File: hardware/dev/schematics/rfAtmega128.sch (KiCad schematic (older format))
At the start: 6 parts

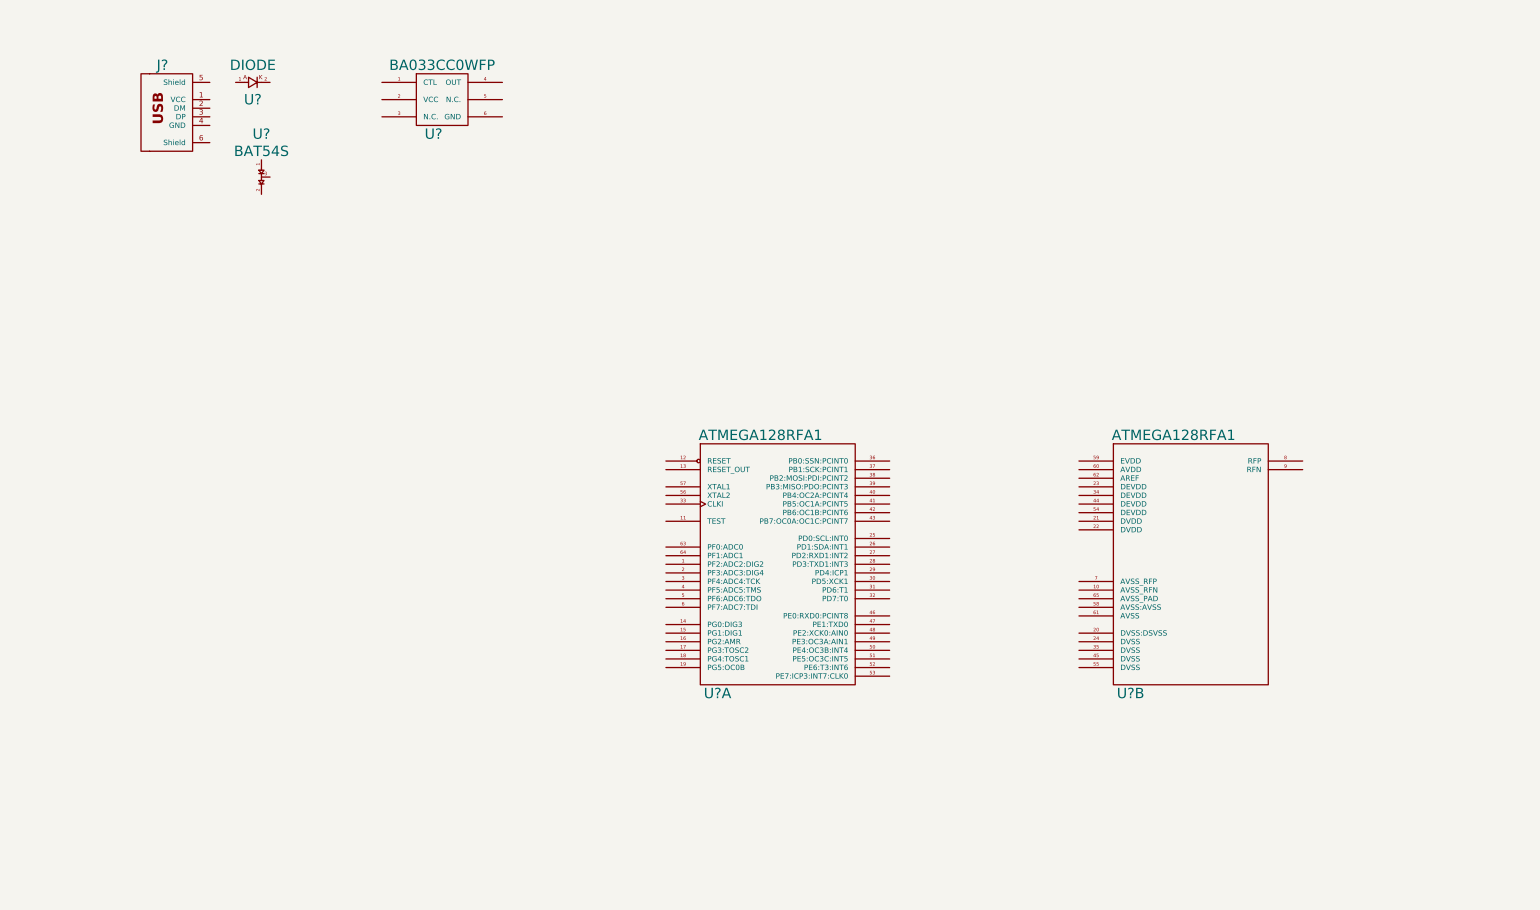
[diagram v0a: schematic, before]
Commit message: New schematic to finish at home.
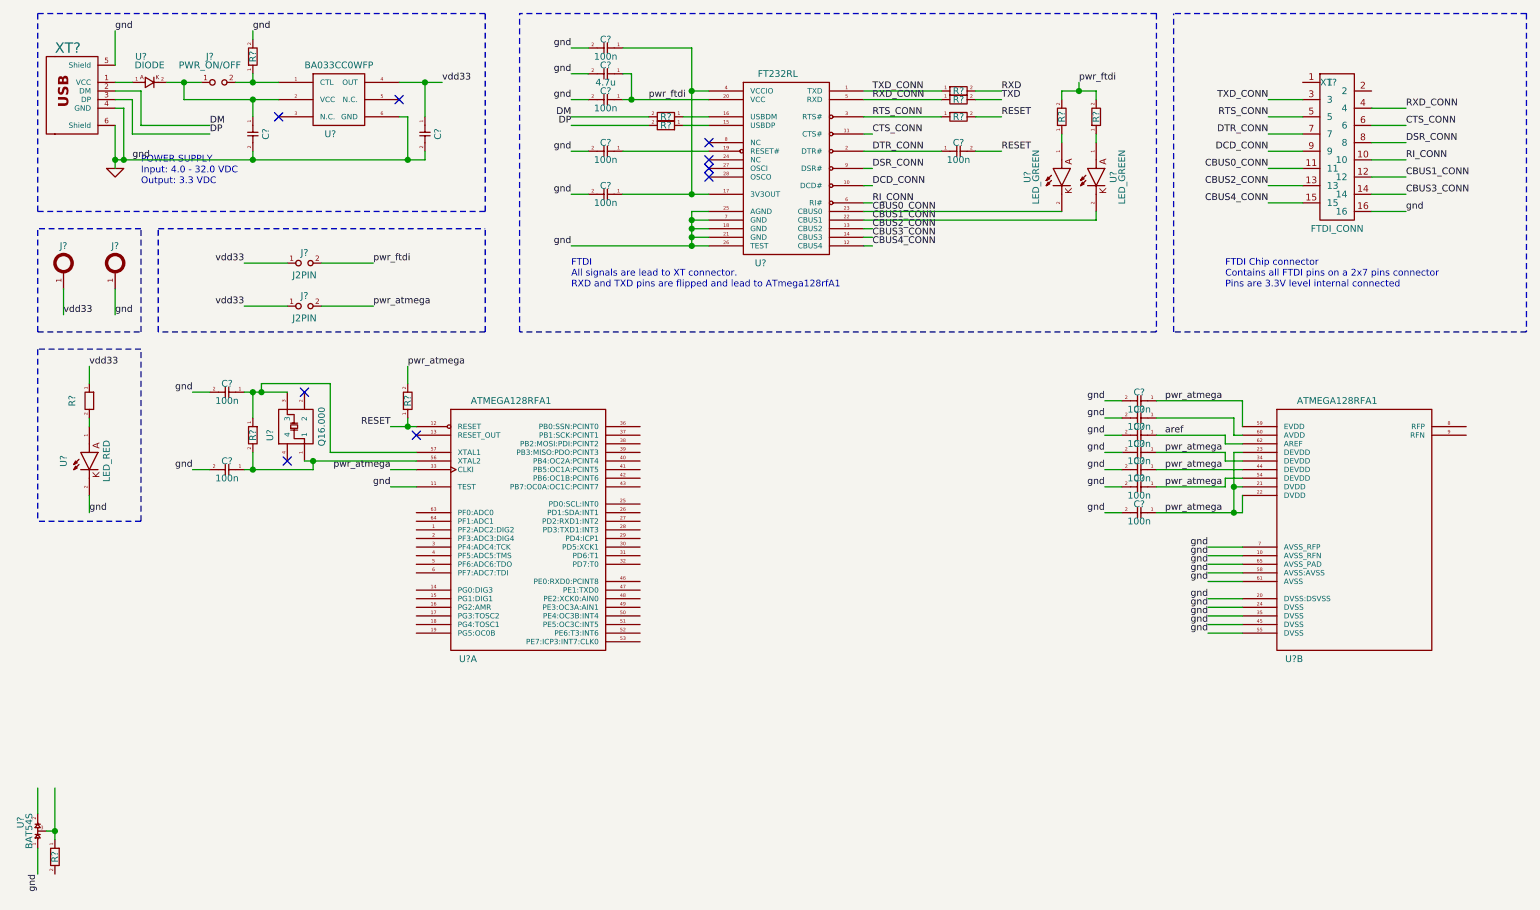
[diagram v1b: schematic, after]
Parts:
- added C?: 330n, symbol CAP_0603
- added C?: 22u, symbol CAP_0603
- added C? (x14): 100n, symbol CAP_0603
- added C?: 4.7u, symbol CAP_0603
- added J?: TEST_VDD33, symbol TEST_PAD
- added J?: TEST_GND, symbol TEST_PAD
- added J? (x2): J2PIN, symbol J2PIN
- added J?: PWR_ON/OFF, symbol J2PIN
- added R? (x12): RES_0603, symbol RES_0603
- added U?: FT232RL, symbol FT232RL
- added U?: LED_RED, symbol LED_RED
- added U? (x2): LED_GREEN, symbol LED_GREEN
- added U?: Q16.000, symbol Q16.000
- added XT?: FTDI_CONN, symbol FTDI_CONN
- gave numbers to parts that had none: 1
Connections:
- net GND: now reaches U?.11 (TEST)
- net GND: now also U?.1, U?.10 (AVSS_RFN), U?.20 (DVSS:DSVSS), U?.24 (DVSS), U?.35 (DVSS), U?.45 (DVSS), U?.55 (DVSS), U?.58 (AVSS:AVSS), U?.6 (GND), U?.61 (AVSS), U?.65 (AVSS_PAD), U?.7 (AVSS_RFP), XT?.4 (GND), XT?.5 (Shield), XT?.6 (Shield), C?.2, C?.2, C?.2, C?.2, C?.2, C?.2, C?.2, C?.2, C?.2, C?.2, C?.2, C?.2, C?.2, C?.2, C?.2, C?.2, J?.1, R?.2, U?.18 (GND), U?.2 (K), U?.21 (GND), U?.25 (AGND), U?.26 (TEST), U?.7 (GND), XT?.16
- net RESET: now reaches U?.12 (RESET)
- net RESET: now also C?.2, R?.1, R?.2
- net pwr_atmega: now reaches U?.33 (CLKI)
- net pwr_atmega: now also U?.21 (DVDD), U?.22 (DVDD), U?.23 (DEVDD), U?.34 (DEVDD), U?.44 (DEVDD), U?.54 (DEVDD), U?.59 (EVDD), C?.1, C?.1, C?.1, C?.1, C?.1, J?.2, R?.2
- net at U?.56 (XTAL2): now also C?.1, R?.2, U?.1
- net at U?.57 (XTAL1): now also C?.1, R?.1, U?.3
- net at U?.60 (AVDD): now also C?.1
- net aref: now reaches U?.62 (AREF)
- net aref: now also C?.1
- net at XT?.1 (VCC): now also U?.1 (A)
- net DM: now reaches XT?.2 (DM)
- net DM: now also R?.2
- net DP: now reaches XT?.3 (DP)
- net DP: now also R?.2
- net at U?.2 (K): now also U?.2 (VCC), C?.1, J?.1
- net at U?.1 (CTL): now also J?.2, R?.1
- net vdd33: now reaches U?.4 (OUT)
- net vdd33: now also C?.1, J?.1, J?.1, J?.1, R?.1
- net at U?.3: now also R?.1
- new net: R?.1, U?.15 (USBDP)
- new net: R?.1, U?.16 (USBDM)
- new net: C?.1, C?.1, U?.17 (3V3OUT), U?.4 (VCCIO)
- new net: C?.1, U?.19 (RESET#)
- new net: R?.2, U?.1 (A)
- new net: R?.1, U?.1 (A) (x2)
- new net CBUS0_CONN: U?.2 (K), U?.23 (CBUS0), XT?.11
- new net CBUS1_CONN: U?.2 (K), U?.22 (CBUS1), XT?.12
- new net CBUS2_CONN: U?.13 (CBUS2), XT?.13
- new net CBUS3_CONN: U?.14 (CBUS3), XT?.14
- new net CBUS4_CONN: U?.12 (CBUS4), XT?.15
- new net CTS_CONN: U?.11 (CTS#), XT?.6
- new net DCD_CONN: U?.10 (DCD#), XT?.9
- new net DSR_CONN: U?.9 (DSR#), XT?.8
- new net DTR_CONN: C?.1, U?.2 (DTR#), XT?.7
- new net RI_CONN: U?.6 (RI#), XT?.10
- new net RTS_CONN: R?.1, U?.3 (RTS#), XT?.5
- new net RXD: R?.2
- new net RXD_CONN: R?.1, U?.5 (RXD), XT?.4
- new net TXD: R?.2
- new net TXD_CONN: R?.1, U?.1 (TXD), XT?.3
- new net pwr_ftdi: C?.1, C?.1, J?.2, R?.2, R?.2, U?.20 (VCC)
- no-connect marks 0 -> 9
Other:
- note added: "FTDI Chip connector\nContains all FTDI pins on a 2x7 pins connector\nPins are 3.3V level internal connected"
- note added: "FTDI\nAll signals are lead to XT connector.\nRXD and TXD pins are flipped and lead to ATmega128rfA1"
- note added: "POWER SUPPLY \nInput: 4.0 - 32.0 VDC\nOutput: 3.3 VDC"
- moved on the sheet: U?, U?A, U?B, XT?
